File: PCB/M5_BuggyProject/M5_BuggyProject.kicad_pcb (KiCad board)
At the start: 2 copper layers, 50.8 x 99.1 mm, 27 parts, among them J1 XT60, J2 VCC, J3 10V, J4 Receiver

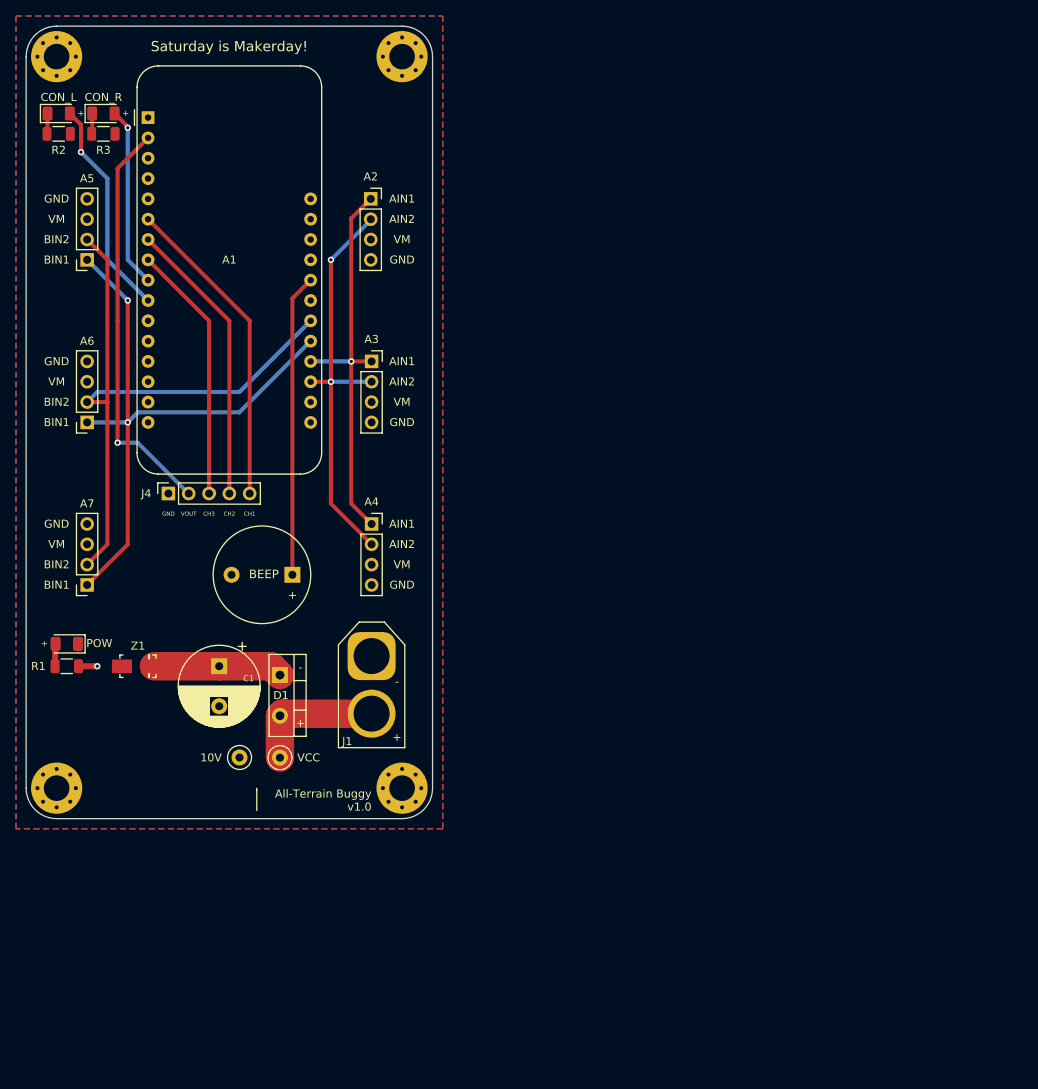
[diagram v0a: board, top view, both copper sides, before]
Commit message: Started PCB v2
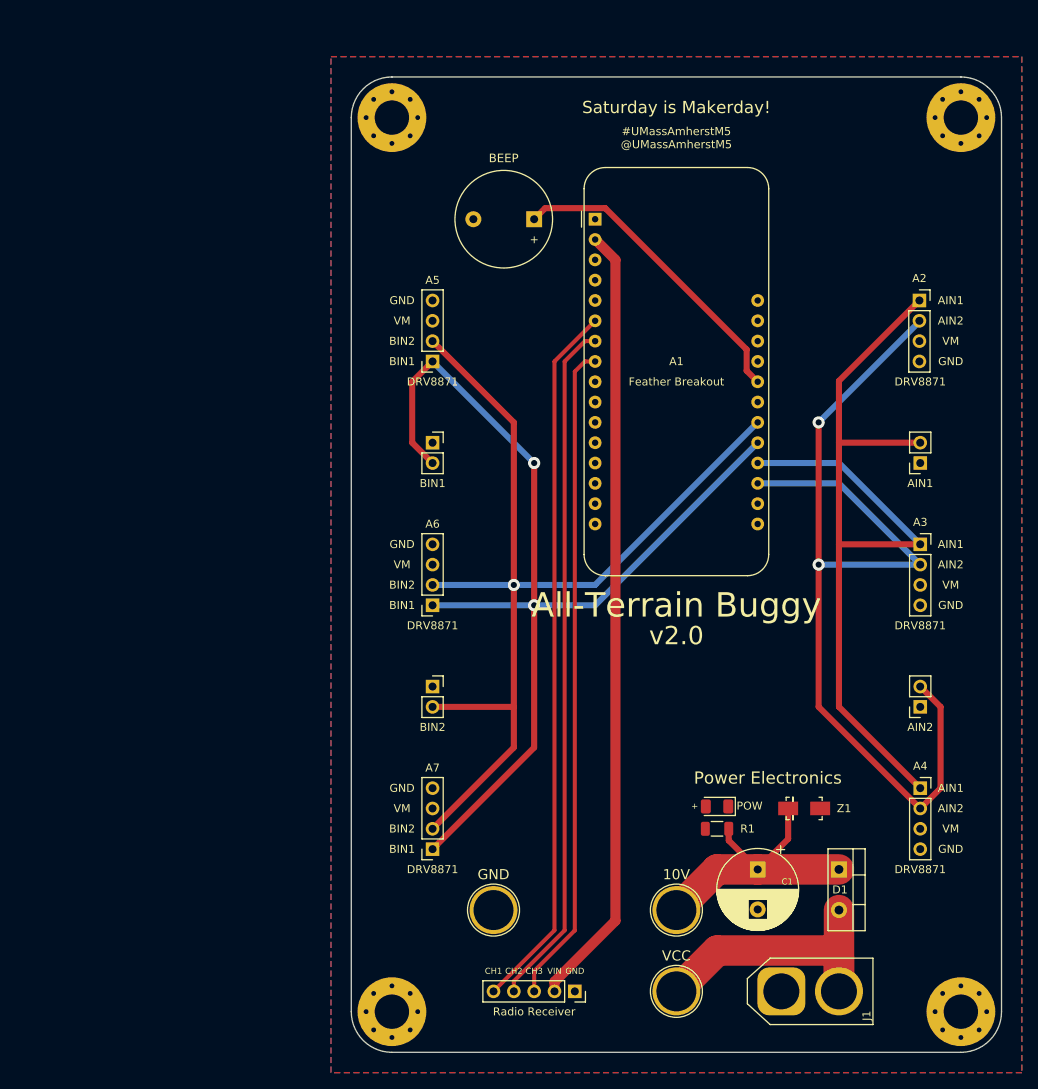
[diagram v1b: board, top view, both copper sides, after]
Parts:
- removed D2, D4: ORANGE, LED_SMD:LED_1206_3216Metric
- removed the G*** at (73.9, 111.1)
- removed R2, R3: 100, Resistor_SMD:R_1206_3216Metric
- added J5: GND, TestPoint:TestPoint_Plated_Hole_D5.0mm, F.Cu at (130.0, 136.9)
- added J6: AIN1, Connector_PinSocket_2.54mm:PinSocket_1x02_P2.54mm_Vertical, F.Cu at (183.4, 81.0)
- added J7: AIN2, Connector_PinSocket_2.54mm:PinSocket_1x02_P2.54mm_Vertical, F.Cu at (183.4, 111.5)
- added J8: BIN1, Connector_PinSocket_2.54mm:PinSocket_1x02_P2.54mm_Vertical, F.Cu at (122.4, 78.5)
- added J9: BIN2, Connector_PinSocket_2.54mm:PinSocket_1x02_P2.54mm_Vertical, F.Cu at (122.4, 109.0)
- H1, H2, H3, H4: footprint MountingHole:MountingHole_3.2mm_M3_Pad_Via -> MountingHole:MountingHole_4.3mm_M4_Pad_Via
- J2, J3: footprint TestPoint:TestPoint_Loop_D1.80mm_Drill1.0mm_Beaded -> TestPoint:TestPoint_Plated_Hole_D5.0mm
- Z1: value Diode -> Zener
- moved H4 116.4 mm to (188.5, 149.6)
- moved Z1 85.2 mm to (168.9, 124.2), turned to 0 degrees
- moved D3 83.8 mm to (158.0, 124.0)
- moved R1 83.8 mm to (158.0, 126.7)
- moved J4 80.3 mm to (140.2, 147.1), turned to 270 degrees
- moved A4 76.1 mm to (183.4, 121.7)
- moved D1 74.0 mm to (173.2, 131.8)
- moved A3 72.3 mm to (183.4, 91.2)
- moved C1 71.9 mm to (163.1, 131.8)
- moved H2 70.3 mm to (188.5, 37.8)
- moved A2 69.7 mm to (183.3, 60.7)
- moved G*** 67.0 mm to (152.9, 111.5)
- moved J1 66.2 mm to (166.0, 147.1), turned to 0 degrees
- moved J3 57.8 mm to (152.9, 136.9)
- moved J2 57.5 mm to (152.9, 147.1)
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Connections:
- A1 pad 10: CONFIG_L -> Net-(A1-Pad10)
- A1 pad 9: CONFIG_R -> Net-(A1-Pad9)
- H1 pad 1: GND -> Net-(H1-Pad1)
- H2 pad 1: GND -> Net-(H2-Pad1)
- H3 pad 1: GND -> Net-(H3-Pad1)
- H4 pad 1: GND -> Net-(H4-Pad1)
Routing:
- net AIN2: track 54.3 -> 126.0 mm
- net AIN1: track 50.3 -> 114.2 mm, vias 1 -> 0
- net BIN1: track 77.0 -> 135.3 mm
- net BIN2: track 77.4 -> 128.6 mm, vias 0 -> 1
- net CHANNEL_2: track 36.0 -> 86.2 mm
- net CHANNEL_3: track 32.6 -> 82.6 mm
- net CHANNEL_1: track 39.6 -> 89.1 mm
- net +3V3: track 51.2 -> 98.2 mm, vias 1 -> 0
- net CONFIG_L: track 27.4 -> 0.00 mm, vias 1 -> 0
- net CONFIG_R: track 22.6 -> 0.00 mm, vias 1 -> 0
- net VCC: track 16.8 -> 37.2 mm
- net +10V: track 18.6 -> 38.2 mm, vias 1 -> 0
- net Net-(D3-Pad2): track 2.82 -> 0.09 mm
- net Net-(D2-Pad1): track 2.65 -> 0.00 mm
- net Net-(D4-Pad1): track 2.57 -> 0.00 mm
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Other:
- board size 50.8 x 99.1 mm -> 81.3 x 121.9 mm
- board text added: "#UMassAmherstM5 @UMassAmherstM5"
- board text added: "All-Terrain Buggy"
- board text added: "DRV8871"
- board text added: "Feather Breakout"
- board text added: "Power Electronics"
- board text added: "Radio Receiver"
- board text added: "VIN"
- board text added: "v2.0"
- board text removed: "#UMassAmherstM5"
- board text removed: "-"
- board text removed: "@UMassAmherstM5"
- board text removed: "All-Terrain Buggy v1.0"
- board text removed: "CON_L"
- board text removed: "CON_R"
- board text removed: "VOUT"
